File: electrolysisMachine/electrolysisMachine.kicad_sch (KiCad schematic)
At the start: 1 part

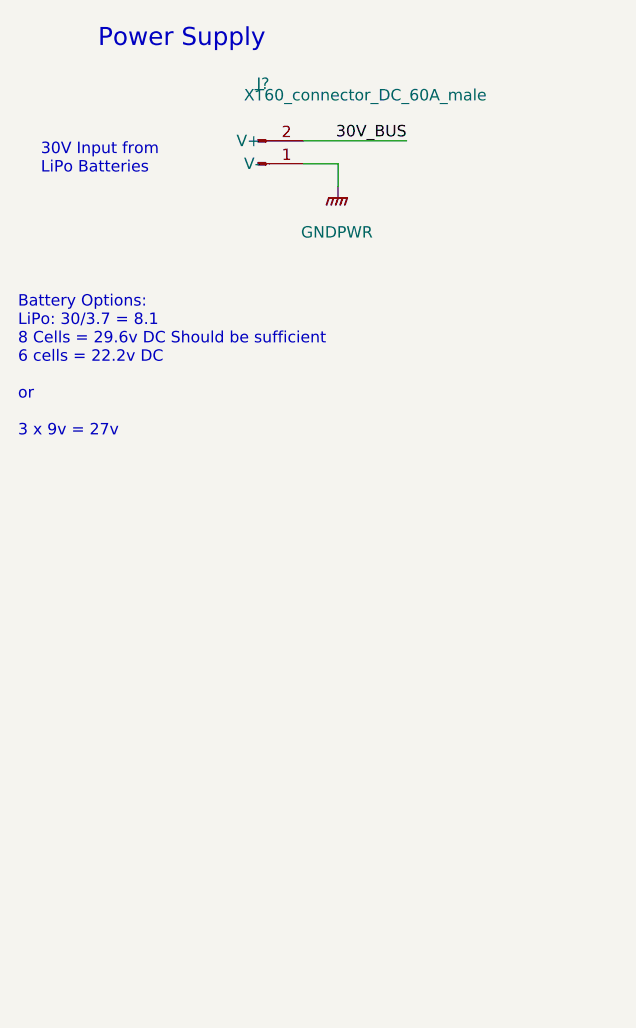
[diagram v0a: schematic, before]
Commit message: started work on shcematic
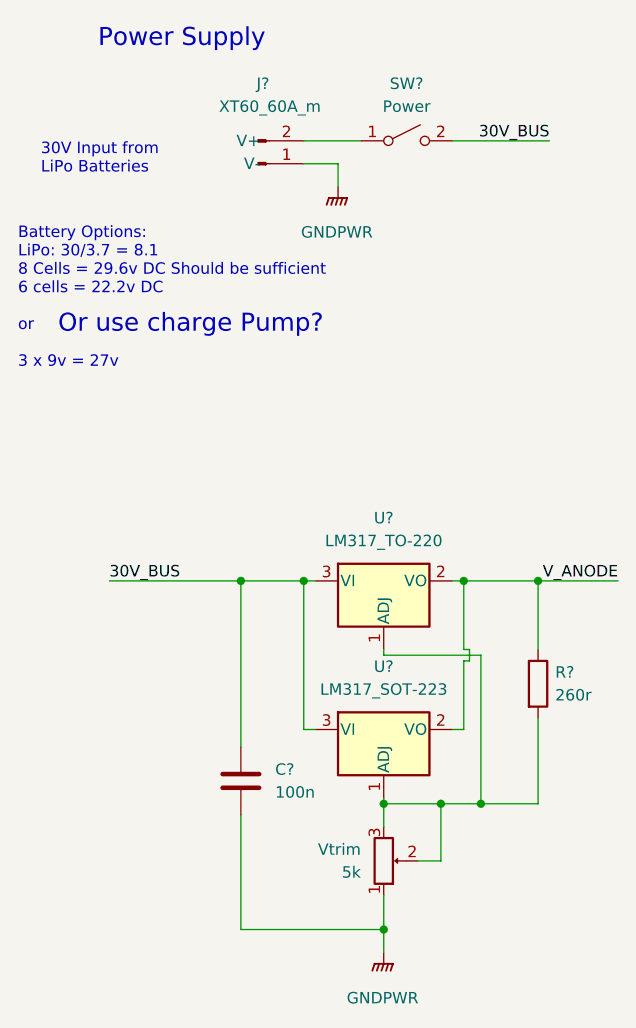
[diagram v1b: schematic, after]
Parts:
- added C?: 100n, Capacitor_SMD:C_0805_2012Metric_Pad1.18x1.45mm_HandSolder, symbol 000_Capacitor_FIlm_Immo:cap_film_0805
- added R?: 260r, Resistor_SMD:R_0805_2012Metric_Pad1.20x1.40mm_HandSolder, symbol 000_Resistors_Immo:Resistor_0805
- added SW?: Power, symbol Switch:SW_SPST
- added U?: LM317_SOT-223, Package_TO_SOT_THT:TO-220-3_Vertical, symbol Regulator_Linear:LM317_SOT-223
- added U?: LM317_TO-220, Package_SO:SOIC-8_3.9x4.9mm_P1.27mm, symbol Regulator_Linear:LM317_TO-220
- added Vtrim: 5k, Potentiometer_THT:Potentiometer_Alps_RK09K_Single_Vertical, symbol Device:R_Potentiometer_Trim
- J?: value XT60_connector_DC_60A_male -> XT60_60A_m
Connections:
- net 30V_BUS: now also C?.1, SW?.2 (B), U?.3 (VI), U?.3 (VI); no longer J?.2 (V+)
- net GNDPWR: now also C?.2, Vtrim.1
- new net: R?.2, U?.1 (ADJ), U?.1 (ADJ), Vtrim.2, Vtrim.3
- new net: J?.2 (V+), SW?.1 (A)
- new net V_ANODE: R?.1, U?.2 (VO), U?.2 (VO)
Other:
- note added: "Or use charge Pump?"
